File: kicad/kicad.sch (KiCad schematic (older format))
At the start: 14 parts, among them J1 Jack-DC, U1 ESP32-DEVKITC-32D, U3 D36V6F3, U4 xL6019

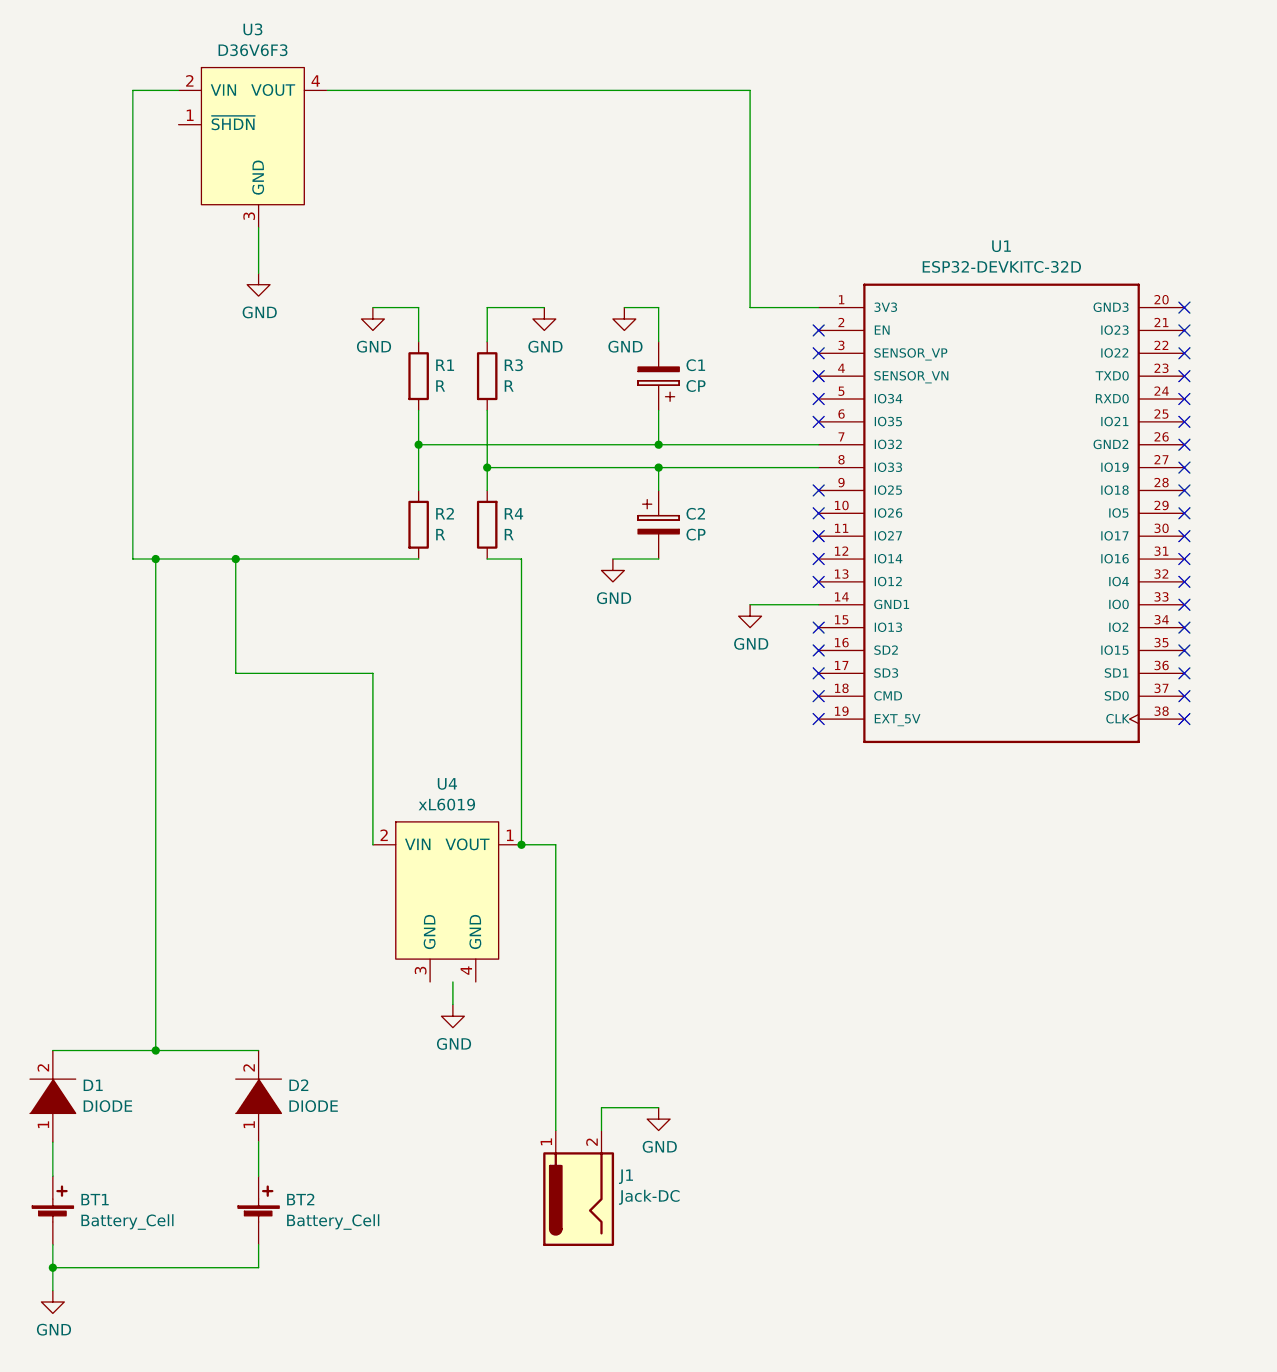
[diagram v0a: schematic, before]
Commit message: Update
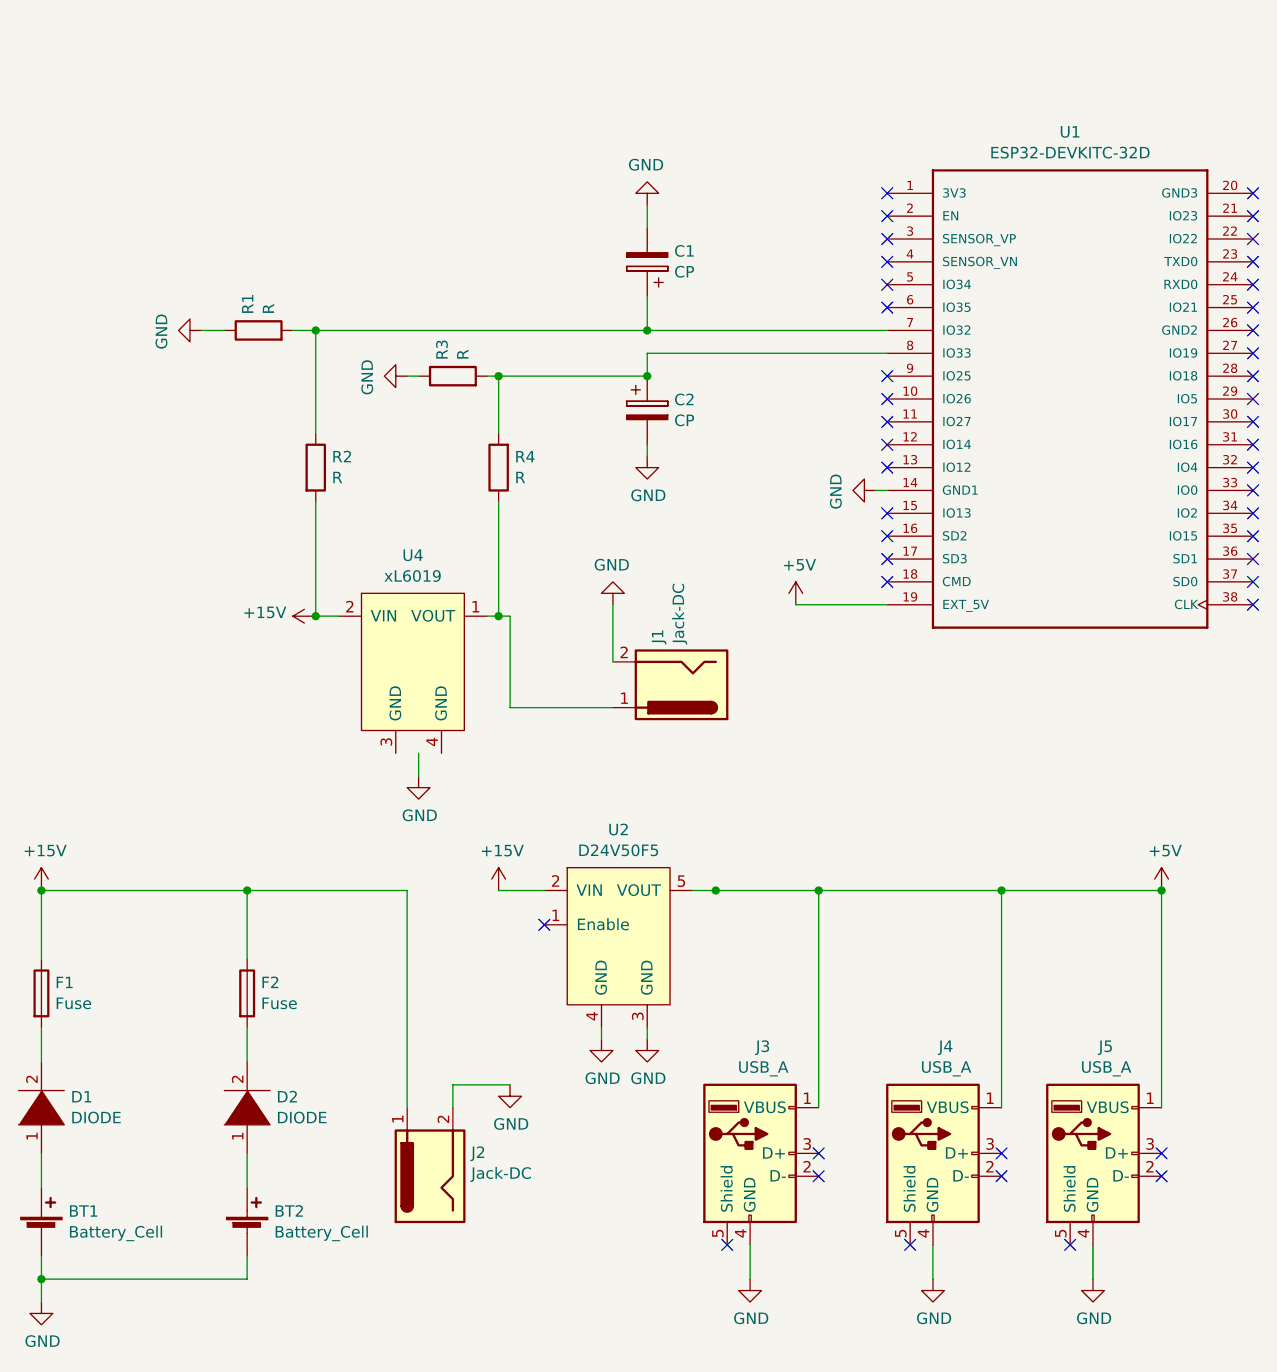
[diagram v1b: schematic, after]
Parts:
- removed U3: D36V6F3, symbol D36V6F3:D36V6F3
- added F1, F2: Fuse, symbol Device:Fuse
- added J2: Jack-DC, symbol Connector:Jack-DC
- added J3, J4, J5: USB_A, symbol Connector:USB_A
- added U2: D24V50F5, symbol D36V6F3:D24V50F5
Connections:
- net GND: now also J2.2, J3.4 (GND), J4.4 (GND), J5.4 (GND), U2.3 (GND), U2.4 (GND)
- net +5V: now reaches U1.19 (EXT_5V)
- net +5V: now also J3.1 (VBUS), J4.1 (VBUS), J5.1 (VBUS), U2.5 (VOUT)
- net +15V: now reaches R2.2, U4.2 (VIN)
- net +15V: now also F1.1, F2.1, J2.1, U2.2 (VIN); no longer D1.2 (A), D2.2 (A)
- new net: D1.2 (A), F1.2
- new net: D2.2 (A), F2.2
- no-connect marks 34 -> 44
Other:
- moved on the sheet: BT1, BT2, C1, C2, D1, D2, J1, R1, R2, R3, R4, U1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

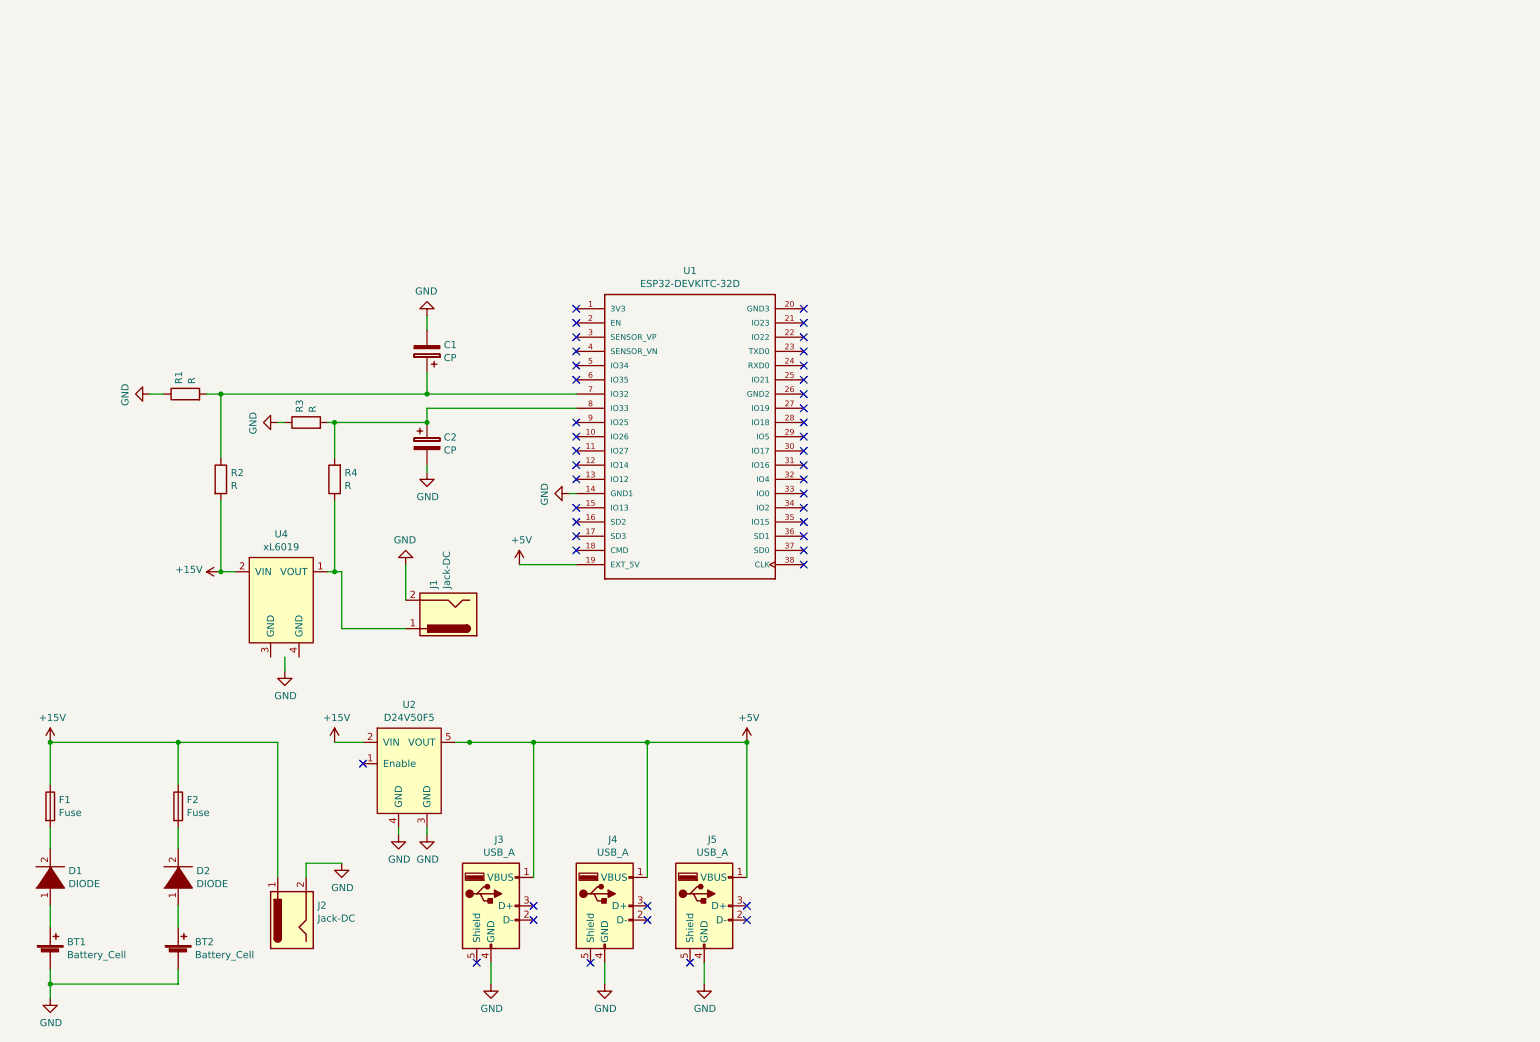
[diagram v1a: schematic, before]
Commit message: Remaining components
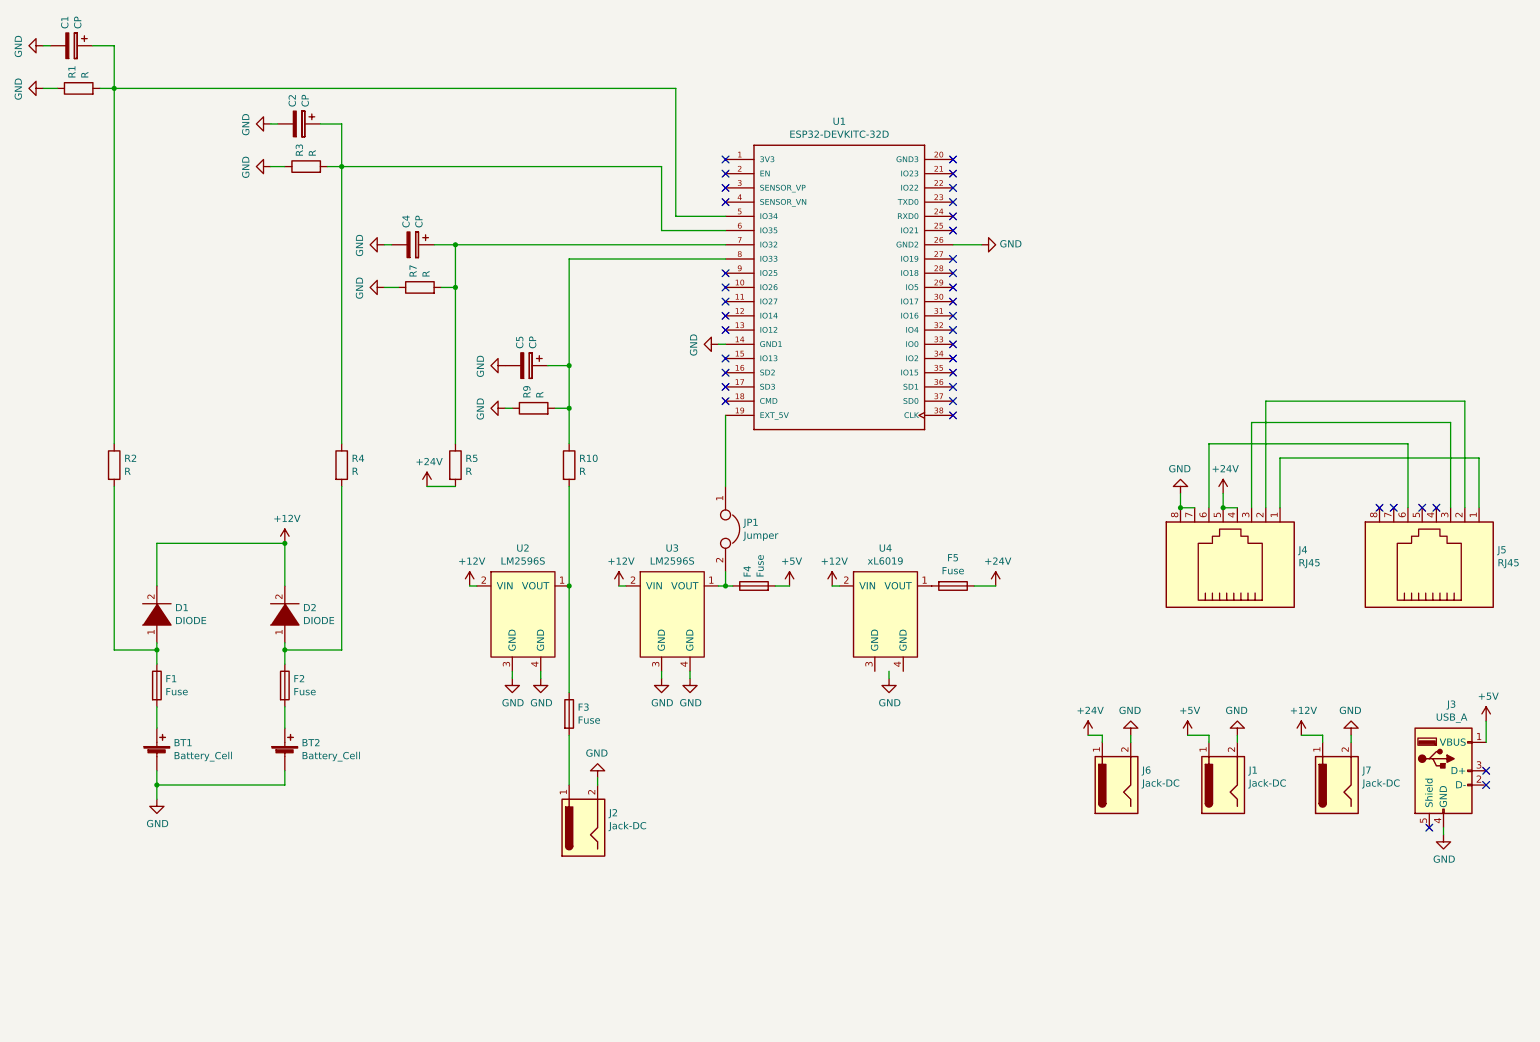
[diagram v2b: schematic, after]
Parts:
- removed J4, J5: USB_A, symbol Connector:USB_A
- removed U2: D24V50F5, symbol D36V6F3:D24V50F5
- added C4, C5: CP, symbol Device:CP
- added F3, F4, F5: Fuse, symbol Device:Fuse
- added J4, J5: RJ45, symbol Connector:RJ45
- added J6, J7: Jack-DC, symbol Connector:Jack-DC
- added JP1: Jumper, symbol Device:Jumper
- added R10, R5, R7, R9: R, symbol Device:R
- added U2, U3: LM2596S, symbol XL60919:LM2596S
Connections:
- net +5V: now also J1.1, F4.2; no longer U1.19 (EXT_5V)
- net GND: now also U1.26 (GND2), C4.2, C5.2, J4.7, J4.8, J6.2, J7.2, R7.1, R9.1, U2.3 (GND), U2.4 (GND), U3.3 (GND), U3.4 (GND)
- net at U1.5 (IO34): now also C1.1, R1.2, R2.1
- net at U1.6 (IO35): now also C2.1, R3.2, R4.1
- net at D1.1 (K): now also F1.1, R2.2; no longer BT1.1 (+)
- net at F1.2: now also BT1.1 (+); no longer D1.2 (A)
- net at D2.1 (K): now also F2.1, R4.2; no longer BT2.1 (+)
- net at F2.2: now also BT2.1 (+); no longer D2.2 (A)
- removed net +15V: F1.1, F2.1, J2.1, R2.2, U4.2 (VIN)
- new net: JP1.1, U1.19 (EXT_5V)
- new net: C4.1, R5.1, R7.2, U1.7 (IO32)
- new net: C5.1, R10.1, R9.2, U1.8 (IO33)
- new net: F3.1, R10.2, U2.1 (VOUT)
- new net: F4.1, JP1.2, U3.1 (VOUT)
- new net: F3.2, J2.1
- new net: F5.2, U4.1 (VOUT)
- new net: J4.1, J5.1
- new net: J4.2, J5.2
- new net: J4.3, J5.3
- new net: J4.6, J5.6
- new net +12V: D1.2 (A), D2.2 (A), J7.1, U2.2 (VIN), U3.2 (VIN), U4.2 (VIN)
- new net +24V: F5.1, J4.4, J4.5, J6.1, R5.2
- no-connect marks 44 -> 38
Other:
- moved on the sheet: BT1, BT2, C1, D1, D2, J1, J2, J3, R1, U1
